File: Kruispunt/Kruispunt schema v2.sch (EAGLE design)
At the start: 122 parts, among them IC1 74ACT132N, IC2 LM555N, IC3 LM555N, IC4 74AC132N, Q1 BC548, Q10 BC548, Q2 2N3906, Q5 BC548, Q6 2N3906, Q9 BC548, X1 Rood2, X10 Voetgagnersknop1, X11 Voetgangersknop 2 en 1, X12 Groen1, X13 Geel1, X14 Groen2, X4 Rood1, X6 Geel2

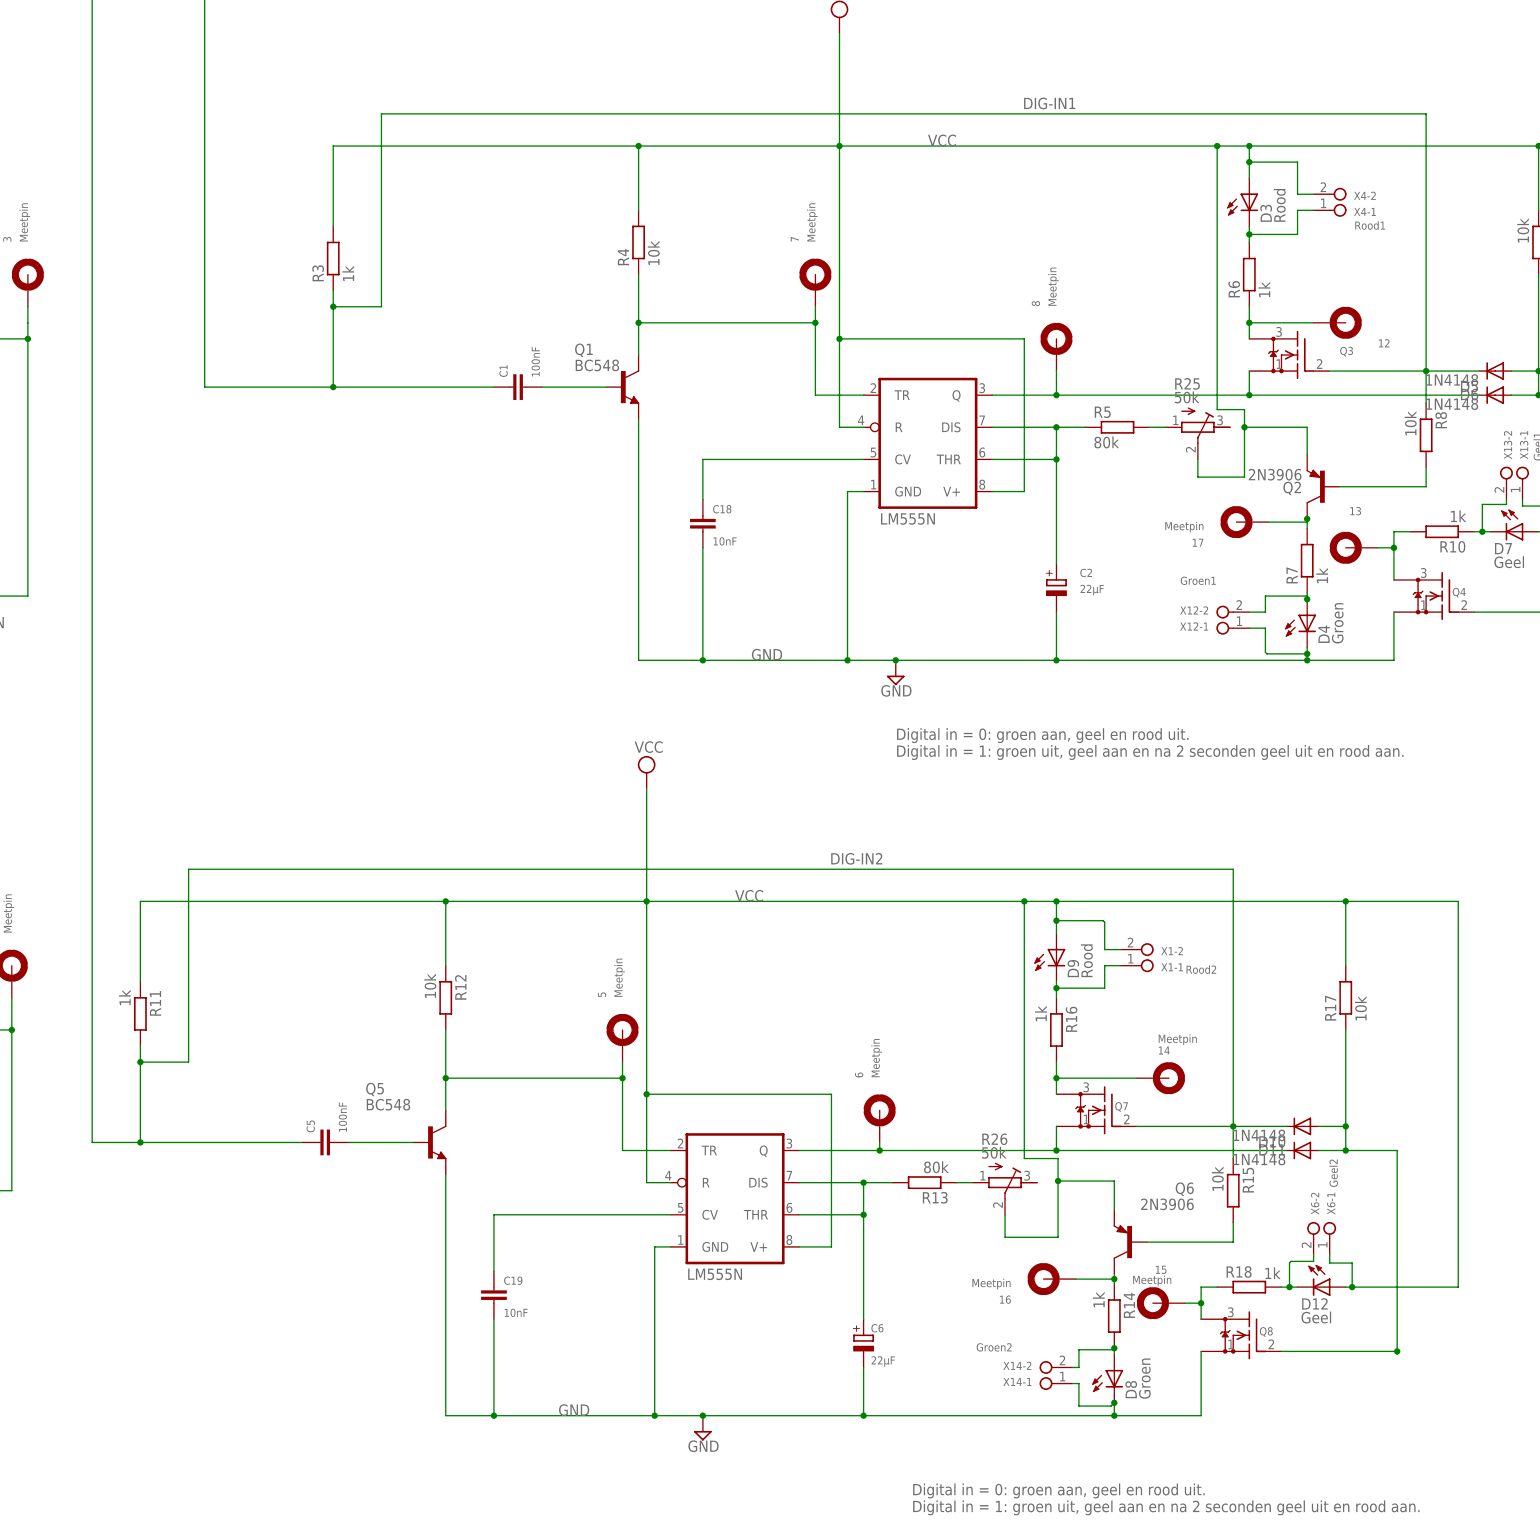
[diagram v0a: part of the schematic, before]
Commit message: v3
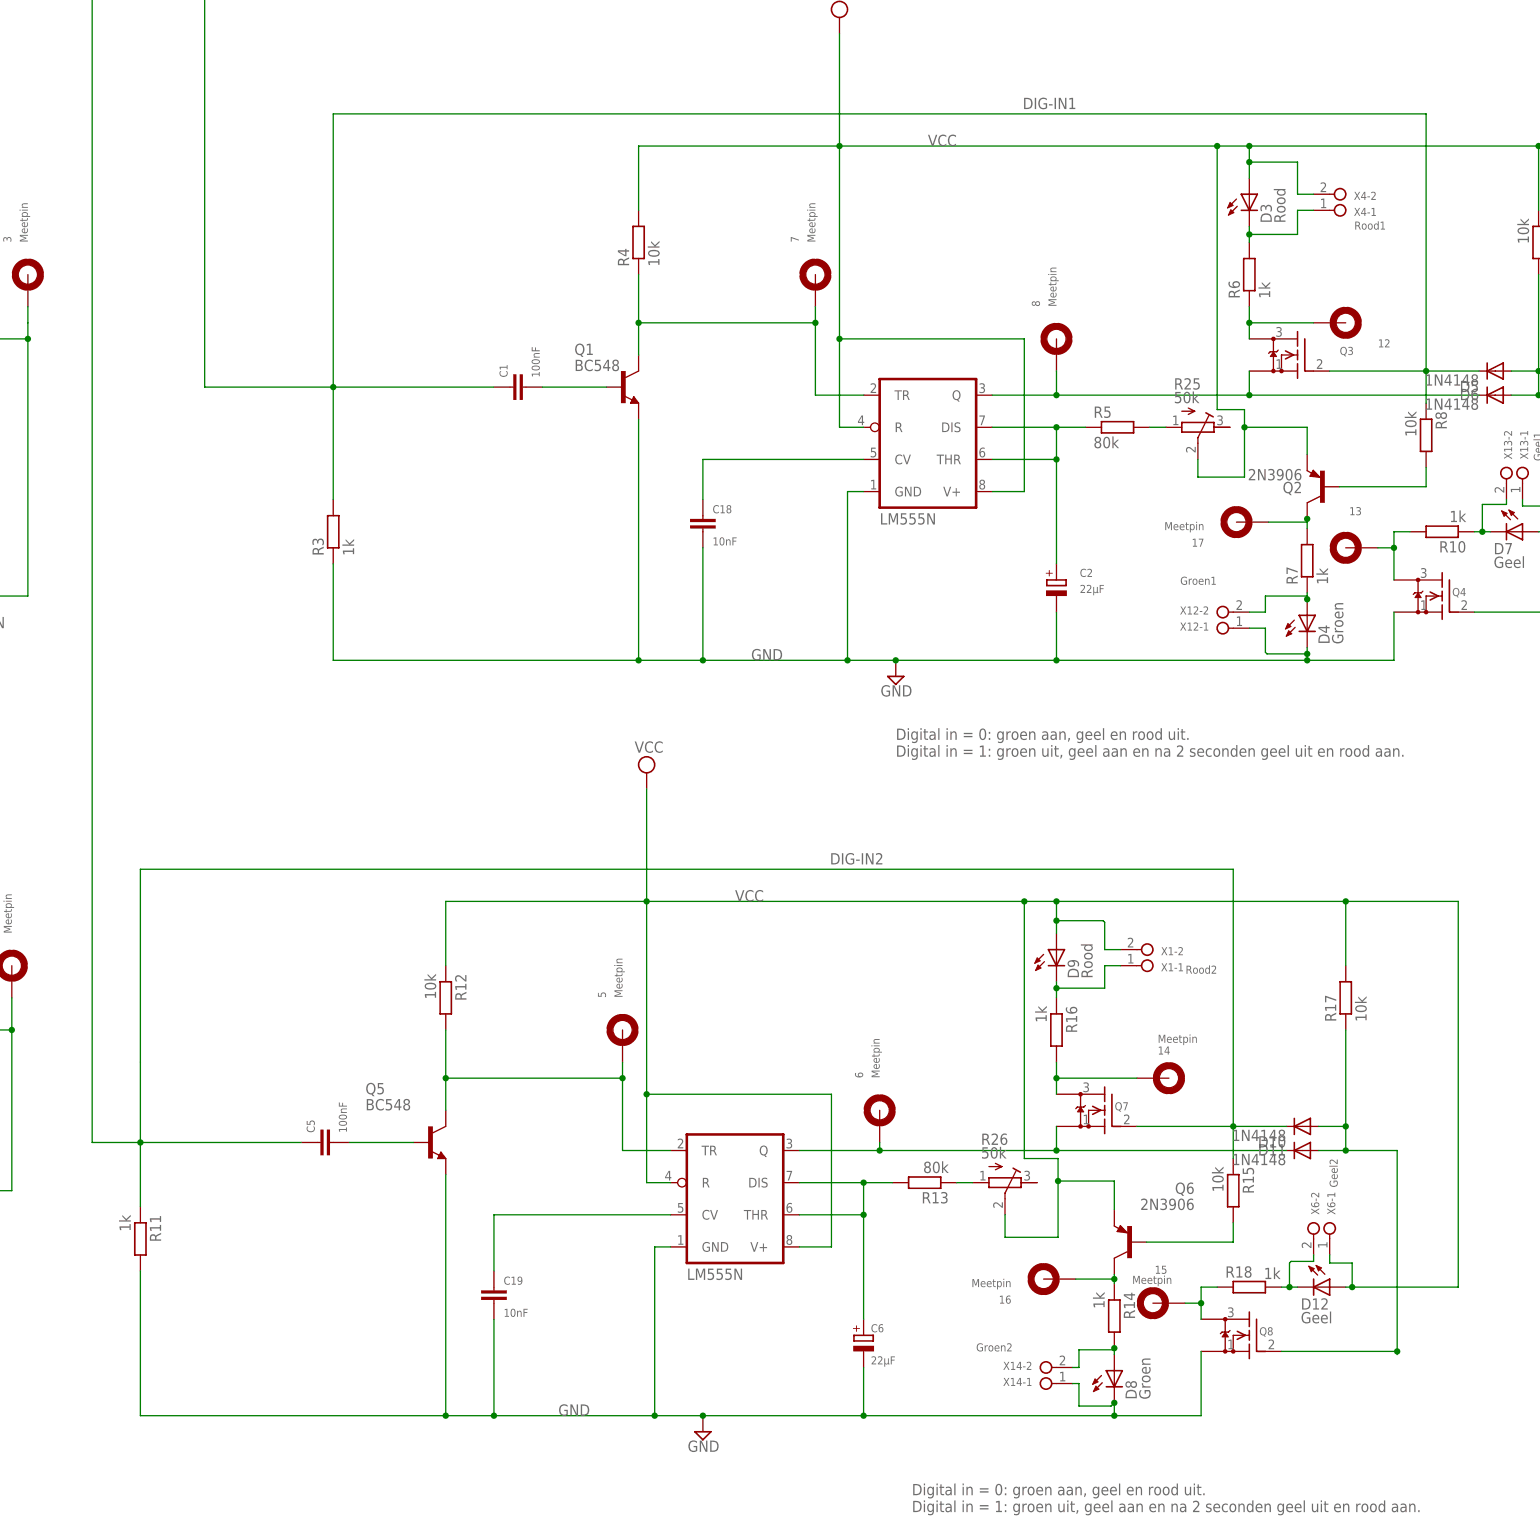
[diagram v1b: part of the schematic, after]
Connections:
- net DIG-IN1: now also R3.2; no longer R3.1
- net DIG-IN2: now also R11.1; no longer R11.2
- net GND: now also R11.2, R3.1
- net VCC: no longer R11.1, R3.2
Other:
- moved on the sheet: R11, R3
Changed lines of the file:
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@@
 <attribute name="VALUE" x="267.462" y="92.71" size="1.778" layer="96" rot="R90"/>
 </instance>
-<instance part="R3" gate="G$1" x="215.9" y="93.98" smashed="yes" rot="R90">
-<attribute name="NAME" x="214.4014" y="90.17" size="1.778" layer="95" rot="R90"/>
-<attribute name="VALUE" x="219.202" y="90.17" size="1.778" layer="96" rot="R90"/>
+<instance part="R3" gate="G$1" x="215.9" y="50.8" smashed="yes" rot="R90">
+<attribute name="NAME" x="214.4014" y="46.99" size="1.778" layer="95" rot="R90"/>
+<attribute name="VALUE" x="219.202" y="46.99" size="1.778" layer="96" rot="R90"/>
 </instance>
 <instance part="R6" gate="G$1" x="360.68" y="91.44" smashed="yes" rot="R90">
@@
 <attribute name="VALUE" x="403.098" y="100.33" size="1.778" layer="96" rot="R270"/>
 </instance>
-<instance part="R11" gate="G$1" x="185.42" y="-25.4" smashed="yes" rot="R270">
-<attribute name="NAME" x="186.9186" y="-21.59" size="1.778" layer="95" rot="R270"/>
-<attribute name="VALUE" x="182.118" y="-21.59" size="1.778" layer="96" rot="R270"/>
+<instance part="R11" gate="G$1" x="185.42" y="-60.96" smashed="yes" rot="R270">
+<attribute name="NAME" x="186.9186" y="-57.15" size="1.778" layer="95" rot="R270"/>
+<attribute name="VALUE" x="182.118" y="-57.15" size="1.778" layer="96" rot="R270"/>
 </instance>
 <instance part="R12" gate="G$1" x="233.68" y="-22.86" smashed="yes" rot="R270">
@@
 <pinref part="X12" gate="-1" pin="P$1"/>
 <wire x1="360.68" y1="35.56" x2="363.22" y2="35.56" width="0.1524" layer="91"/>
+<pinref part="R3" gate="G$1" pin="1"/>
+<wire x1="215.9" y1="45.72" x2="215.9" y2="30.48" width="0.1524" layer="91"/>
+<wire x1="215.9" y1="30.48" x2="264.16" y2="30.48" width="0.1524" layer="91"/>
+<junction x="264.16" y="30.48"/>
 </segment>
 <segment>
@@
 <pinref part="X14" gate="-1" pin="P$1"/>
 <wire x1="332.74" y1="-83.82" x2="333.756" y2="-83.82" width="0.1524" layer="91"/>
+<pinref part="R11" gate="G$1" pin="2"/>
+<wire x1="185.42" y1="-66.04" x2="185.42" y2="-88.9" width="0.1524" layer="91"/>
+<wire x1="185.42" y1="-88.9" x2="233.68" y2="-88.9" width="0.1524" layer="91"/>
+<junction x="233.68" y="-88.9"/>
 </segment>
 <segment>
@@
 <net name="VCC" class="1">
 <segment>
-<wire x1="215.9" y1="99.06" x2="215.9" y2="111.76" width="0.1524" layer="91"/>
-<wire x1="215.9" y1="111.76" x2="264.16" y2="111.76" width="0.1524" layer="91"/>
 <wire x1="264.16" y1="111.76" x2="264.16" y2="101.6" width="0.1524" layer="91"/>
 <pinref part="SUPPLY3" gate="G$1" pin="VCC"/>
 <wire x1="295.91" y1="129.54" x2="295.91" y2="111.76" width="0.1524" layer="91"/>
 <wire x1="295.91" y1="111.76" x2="264.16" y2="111.76" width="0.1524" layer="91"/>
-<junction x="264.16" y="111.76"/>
 <pinref part="IC2" gate="A" pin="V+"/>
 <wire x1="320.04" y1="57.15" x2="325.12" y2="57.15" width="0.1524" layer="91"/>
@@
 <wire x1="360.68" y1="106.68" x2="360.68" y2="109.22" width="0.1524" layer="91"/>
 <label x="309.88" y="111.76" size="1.778" layer="95"/>
-<pinref part="R3" gate="G$1" pin="2"/>
 <pinref part="R4" gate="G$1" pin="2"/>
 <wire x1="360.68" y1="109.22" x2="360.68" y2="111.76" width="0.1524" layer="91"/>
@@
 </segment>
 <segment>
-<wire x1="185.42" y1="-20.32" x2="185.42" y2="-7.62" width="0.1524" layer="91"/>
-<wire x1="185.42" y1="-7.62" x2="233.68" y2="-7.62" width="0.1524" layer="91"/>
 <wire x1="233.68" y1="-7.62" x2="233.68" y2="-17.78" width="0.1524" layer="91"/>
 <pinref part="SUPPLY4" gate="G$1" pin="VCC"/>
 <wire x1="265.43" y1="10.16" x2="265.43" y2="-7.62" width="0.1524" layer="91"/>
 <wire x1="265.43" y1="-7.62" x2="233.68" y2="-7.62" width="0.1524" layer="91"/>
-<junction x="233.68" y="-7.62"/>
 <pinref part="IC3" gate="A" pin="V+"/>
 <wire x1="289.56" y1="-62.23" x2="294.64" y2="-62.23" width="0.1524" layer="91"/>
@@
 <wire x1="330.2" y1="-12.7" x2="330.2" y2="-10.668" width="0.1524" layer="91"/>
 <label x="279.4" y="-7.62" size="1.778" layer="95"/>
-<pinref part="R11" gate="G$1" pin="1"/>
 <pinref part="R12" gate="G$1" pin="1"/>
 <wire x1="330.2" y1="-10.668" x2="330.2" y2="-7.62" width="0.1524" layer="91"/>
@@
 <segment>
 <wire x1="177.8" y1="-45.72" x2="185.42" y2="-45.72" width="0.1524" layer="91"/>
-<wire x1="185.42" y1="-30.48" x2="185.42" y2="-33.02" width="0.1524" layer="91"/>
 <junction x="185.42" y="-45.72"/>
 <wire x1="185.42" y1="-33.02" x2="185.42" y2="-45.72" width="0.1524" layer="91"/>
-<wire x1="185.42" y1="-33.02" x2="193.04" y2="-33.02" width="0.1524" layer="91"/>
-<junction x="185.42" y="-33.02"/>
-<wire x1="193.04" y1="-33.02" x2="193.04" y2="-2.54" width="0.1524" layer="91"/>
-<wire x1="193.04" y1="-2.54" x2="358.14" y2="-2.54" width="0.1524" layer="91"/>
+<wire x1="185.42" y1="-33.02" x2="185.42" y2="-2.54" width="0.1524" layer="91"/>
+<wire x1="185.42" y1="-2.54" x2="358.14" y2="-2.54" width="0.1524" layer="91"/>
 <wire x1="358.14" y1="-2.54" x2="358.14" y2="-43.18" width="0.1524" layer="91"/>
 <wire x1="358.14" y1="-43.18" x2="358.14" y2="-48.26" width="0.1524" layer="91"/>
@@
 <pinref part="Q7" gate="G$1" pin="G"/>
 <wire x1="342.9" y1="-43.18" x2="358.14" y2="-43.18" width="0.1524" layer="91"/>
-<pinref part="R11" gate="G$1" pin="2"/>
 <pinref part="R15" gate="G$1" pin="1"/>
 <pinref part="D11" gate="G$1" pin="C"/>
@@
 <wire x1="185.42" y1="152.4" x2="177.8" y2="152.4" width="0.1524" layer="91"/>
 <wire x1="177.8" y1="152.4" x2="177.8" y2="-45.72" width="0.1524" layer="91"/>
+<pinref part="R11" gate="G$1" pin="1"/>
+<wire x1="185.42" y1="-55.88" x2="185.42" y2="-45.72" width="0.1524" layer="91"/>
 </segment>
 </net>
@@
 <net name="DIG-IN1" class="0">
 <segment>
-<wire x1="215.9" y1="88.9" x2="215.9" y2="86.36" width="0.1524" layer="91"/>
-<wire x1="215.9" y1="86.36" x2="215.9" y2="73.66" width="0.1524" layer="91"/>
-<wire x1="215.9" y1="86.36" x2="223.52" y2="86.36" width="0.1524" layer="91"/>
-<junction x="215.9" y="86.36"/>
-<wire x1="223.52" y1="86.36" x2="223.52" y2="116.84" width="0.1524" layer="91"/>
-<wire x1="223.52" y1="116.84" x2="388.62" y2="116.84" width="0.1524" layer="91"/>
+<wire x1="215.9" y1="73.66" x2="215.9" y2="116.84" width="0.1524" layer="91"/>
+<wire x1="215.9" y1="116.84" x2="388.62" y2="116.84" width="0.1524" layer="91"/>
 <wire x1="388.62" y1="116.84" x2="388.62" y2="76.2" width="0.1524" layer="91"/>
 <junction x="388.62" y="76.2"/>
@@
 <pinref part="Q3" gate="G$1" pin="G"/>
 <wire x1="373.38" y1="76.2" x2="388.62" y2="76.2" width="0.1524" layer="91"/>
-<pinref part="R3" gate="G$1" pin="1"/>
 <wire x1="215.9" y1="73.66" x2="195.58" y2="73.66" width="0.1524" layer="91"/>
 <junction x="215.9" y="73.66"/>
@@
 <wire x1="203.2" y1="152.4" x2="195.58" y2="152.4" width="0.1524" layer="91"/>
 <wire x1="195.58" y1="152.4" x2="195.58" y2="73.66" width="0.1524" layer="91"/>
-</segment>
-</net>
+<pinref part="R3" gate="G$1" pin="2"/>
+<wire x1="215.9" y1="55.88" x2="215.9" y2="73.66" width="0.1524" layer="91"/>
+</segment>
+</net>
